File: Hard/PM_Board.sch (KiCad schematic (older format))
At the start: 63 parts, among them J1 Micro_SD_Card_Det_Hirose_DM3AT, J101 LiPo_V+, J102 LiPo_V-, J2 KRC_Conn_SWD, J3 USB_B_Micro, J4 KRC_Conn_CAN, J5 KRC_Conn_CAN, J6 KRC_Conn_CAN, Q1 SSM6J501NU, Q2 2n7002, U1 CY8C58xxLTI-LPxxx, U2 INA226, U3 NCV7342, Y1 24MHz

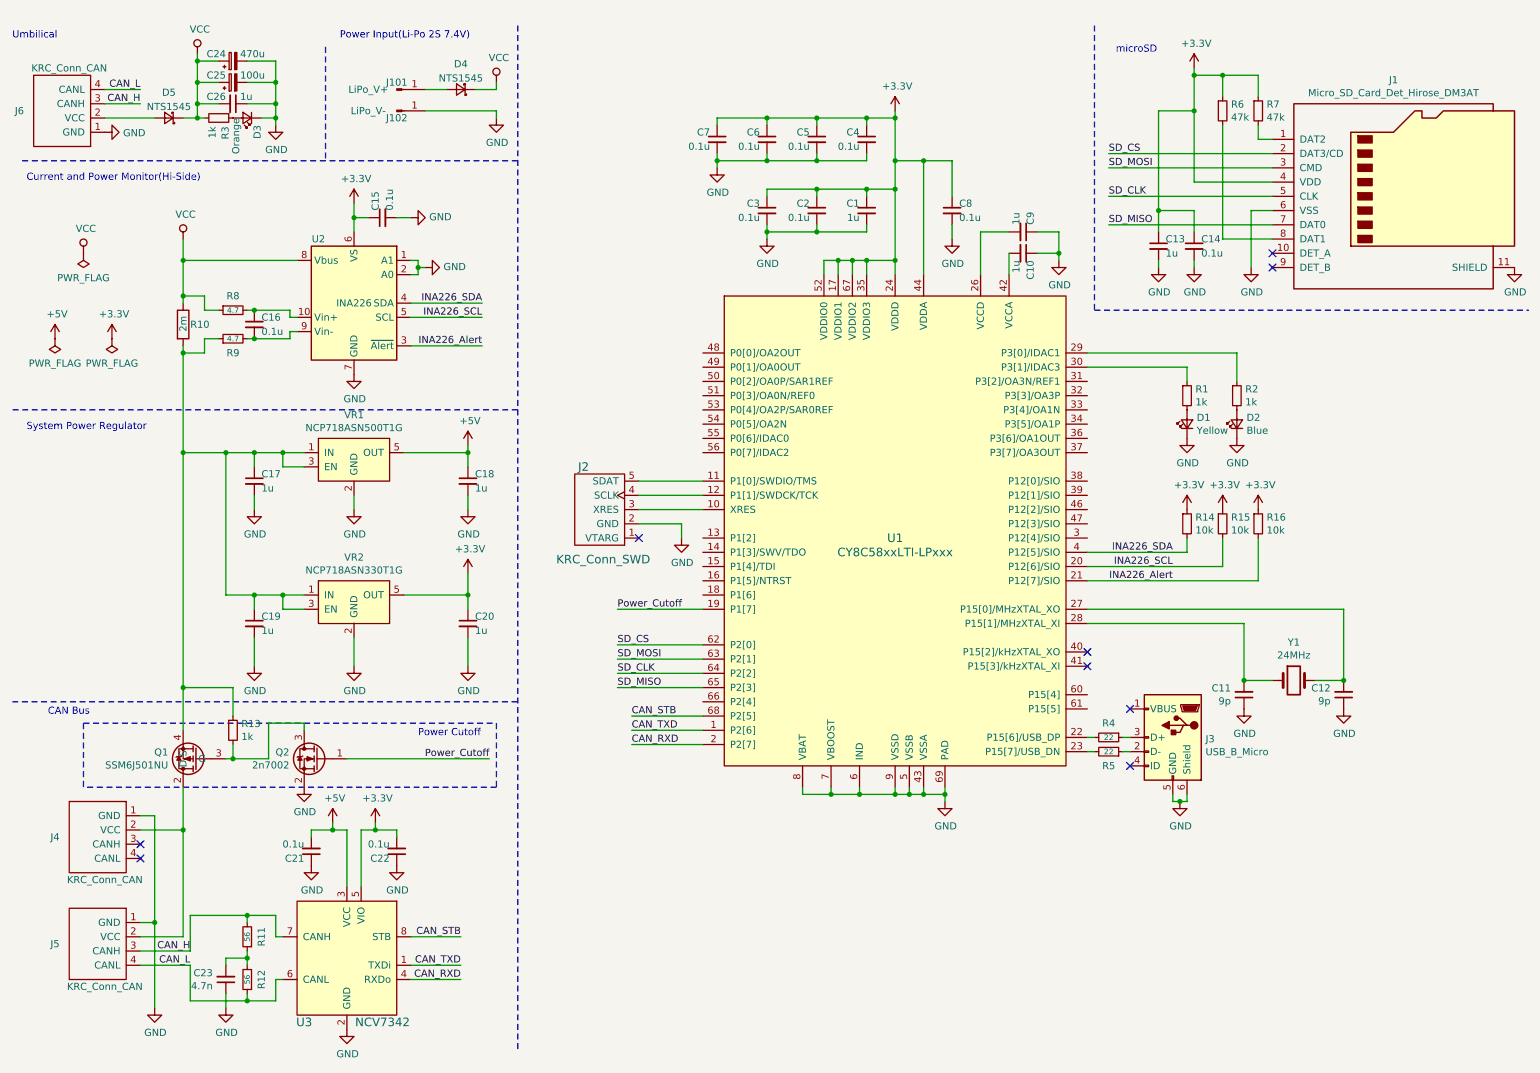
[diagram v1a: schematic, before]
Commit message: [add] 配線中だよ
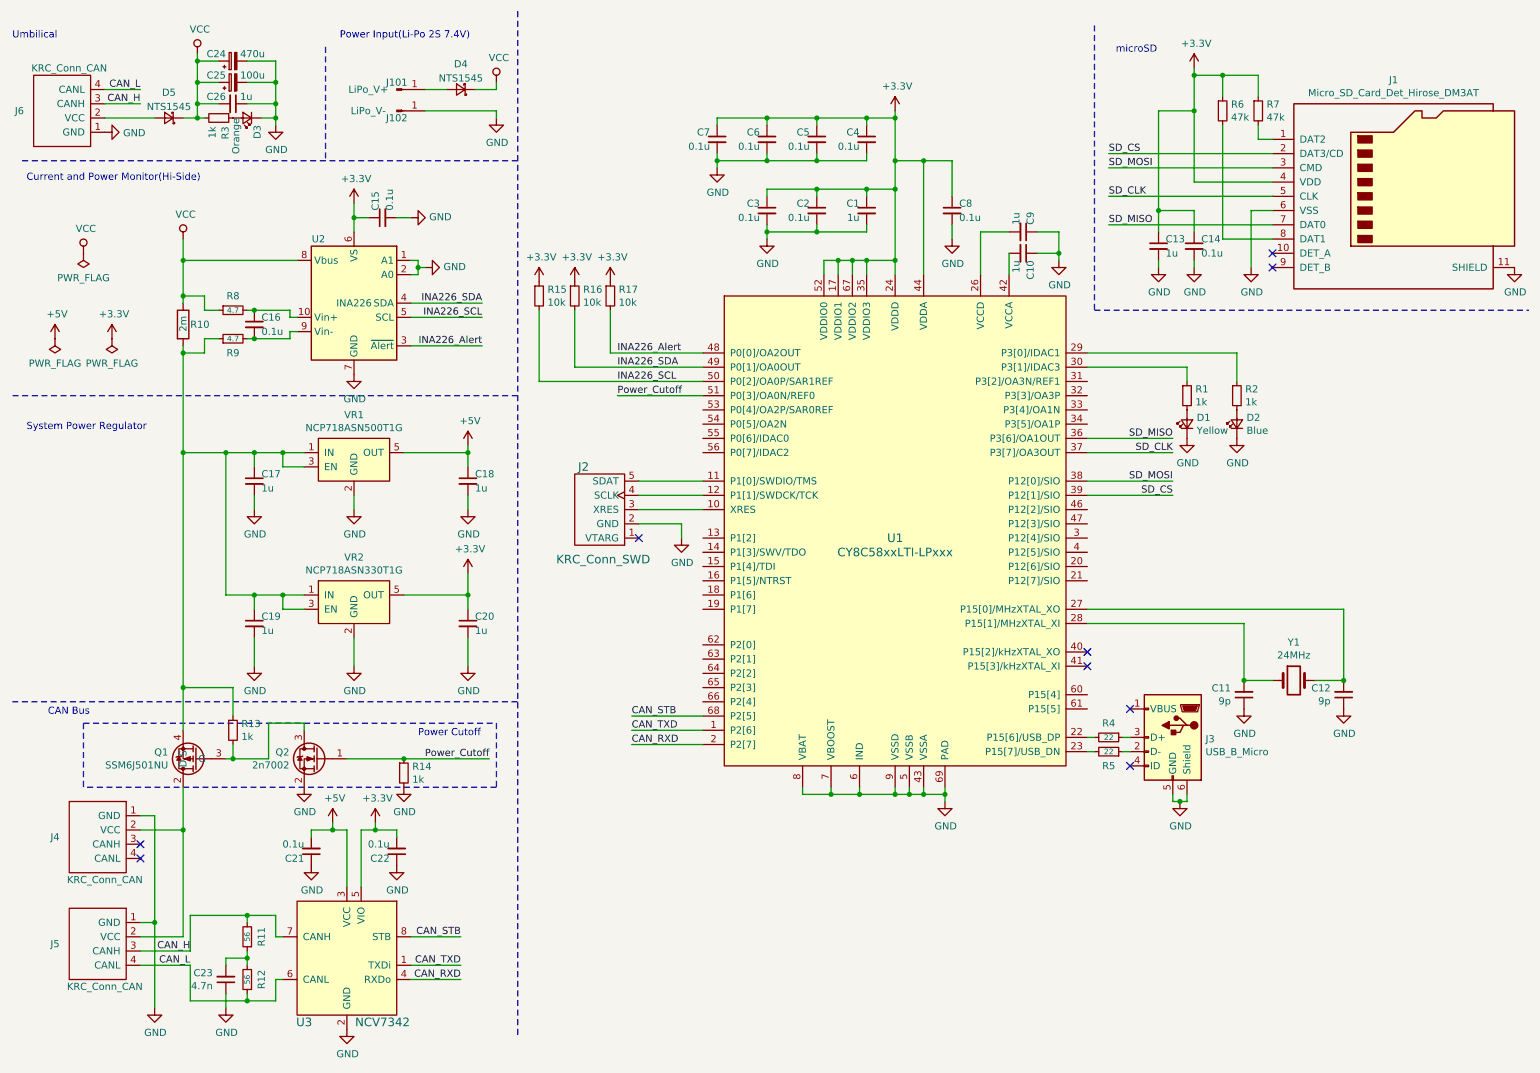
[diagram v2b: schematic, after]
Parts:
- added R14: 1k, Resistor_SMD:R_0402_1005Metric, symbol Device:R_Small
- renumbered R14 to R15, R15 to R16, R16 to R17
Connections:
- net GND: now also R14.2
- net INA226_Alert: now also U1.48 (P0[0]/OA2OUT); no longer U1.21 (P12[7]/SIO)
- net INA226_SCL: now also R15.2, U1.50 (P0[2]/OA0P/SAR1REF); no longer R16.2, U1.20 (P12[6]/SIO)
- net INA226_SDA: now also R16.2, U1.49 (P0[1]/OA0OUT); no longer R15.2, U1.4 (P12[5]/SIO)
- net Power_Cutoff: now also U1.51 (P0[3]/OA0N/REF0), R14.1; no longer U1.19 (P1[7])
- net SD_CLK: now also U1.37 (P3[7]/OA3OUT); no longer U1.64 (P2[2])
- net SD_CS: now also U1.39 (P12[1]/SIO); no longer U1.62 (P2[0])
- net SD_MISO: now also U1.36 (P3[6]/OA1OUT); no longer U1.65 (P2[3])
- net SD_MOSI: now also U1.38 (P12[0]/SIO); no longer U1.63 (P2[1])
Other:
- moved on the sheet: R15, R16, R17
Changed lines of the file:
@@
 	1500 6050 1500 6800
 Wire Notes Line
-	4050 500  4050 7700
+	4050 400  4050 7600
 Wire Notes Line
 	4050 1450 550  1450
@@
 Connection ~ 3700 3500
 Wire Notes Line
-	4050 3200 500  3200
+	4050 3100 500  3100
 Wire Notes Line
 	500  5250 4050 5250
@@
 Wire Wire Line
 	4850 5550 5350 5550
-Text Label 4750 5150 0    50   ~ 0
+Text Label 8650 3400 2    50   ~ 0
 SD_MISO
-Text Label 4750 5050 0    50   ~ 0
+Text Label 8650 3500 2    50   ~ 0
 SD_CLK
-Text Label 4750 4950 0    50   ~ 0
+Text Label 8650 3700 2    50   ~ 0
 SD_MOSI
-Text Label 4750 4850 0    50   ~ 0
+Text Label 8650 3800 2    50   ~ 0
 SD_CS
 Wire Wire Line
-	4750 4850 5350 4850
-Wire Wire Line
-	4750 4950 5350 4950
-Wire Wire Line
-	4750 5050 5350 5050
-Wire Wire Line
-	4750 5150 5350 5150
+	8650 3800 8050 3800
+Wire Wire Line
+	8650 3700 8050 3700
+Wire Wire Line
+	8650 3500 8050 3500
+Wire Wire Line
+	8650 3400 8050 3400
 Text Label 3800 2450 2    50   ~ 0
 INA226_SDA
@@
 Wire Wire Line
 	3300 2550 3800 2550
-Text Label 8650 4200 2    50   ~ 0
+Text Label 4750 2900 0    50   ~ 0
 INA226_SDA
-Text Label 8650 4300 2    50   ~ 0
+Text Label 4750 3000 0    50   ~ 0
 INA226_SCL
-Text Label 8650 4400 2    50   ~ 0
+Text Label 4750 2800 0    50   ~ 0
 INA226_Alert
 Wire Wire Line
-	8050 4200 8750 4200
-Wire Wire Line
-	9000 4300 9000 4100
-Wire Wire Line
-	8050 4300 9000 4300
-Wire Wire Line
-	8750 4100 8750 4200
-Wire Wire Line
-	9250 4400 9250 4100
-Wire Wire Line
-	8050 4400 9250 4400
+	4700 2800 4700 2500
 $Comp
 L power:+3.3V #PWR0137
 U 1 1 5D91E91D
-P 8750 3900
-F 0 "#PWR0137" H 8750 3750 50  0001 C CNN
-F 1 "+3.3V" H 8765 4073 50  0000 C CNN
-F 2 "" H 8750 3900 50  0001 C CNN
-F 3 "" H 8750 3900 50  0001 C CNN
-	1    8750 3900
+P 4200 2300
+F 0 "#PWR0137" H 4200 2150 50  0001 C CNN
+F 1 "+3.3V" H 4215 2473 50  0000 C CNN
+F 2 "" H 4200 2300 50  0001 C CNN
+F 3 "" H 4200 2300 50  0001 C CNN
+	1    4200 2300
 	1    0    0    -1
 $EndComp
@@
 L power:+3.3V #PWR0138
 U 1 1 5D91E993
-P 9000 3900
-F 0 "#PWR0138" H 9000 3750 50  0001 C CNN
-F 1 "+3.3V" H 9015 4073 50  0000 C CNN
-F 2 "" H 9000 3900 50  0001 C CNN
-F 3 "" H 9000 3900 50  0001 C CNN
-	1    9000 3900
+P 4450 2300
+F 0 "#PWR0138" H 4450 2150 50  0001 C CNN
+F 1 "+3.3V" H 4465 2473 50  0000 C CNN
+F 2 "" H 4450 2300 50  0001 C CNN
+F 3 "" H 4450 2300 50  0001 C CNN
+	1    4450 2300
 	1    0    0    -1
 $EndComp
@@
 L power:+3.3V #PWR0139
 U 1 1 5D91EA02
-P 9250 3900
-F 0 "#PWR0139" H 9250 3750 50  0001 C CNN
-F 1 "+3.3V" H 9265 4073 50  0000 C CNN
-F 2 "" H 9250 3900 50  0001 C CNN
-F 3 "" H 9250 3900 50  0001 C CNN
-	1    9250 3900
+P 4700 2300
+F 0 "#PWR0139" H 4700 2150 50  0001 C CNN
+F 1 "+3.3V" H 4715 2473 50  0000 C CNN
+F 2 "" H 4700 2300 50  0001 C CNN
+F 3 "" H 4700 2300 50  0001 C CNN
+	1    4700 2300
 	1    0    0    -1
 $EndComp
@@
 Wire Wire Line
 	6900 1450 7100 1450
-Text Label 4750 4600 0    50   ~ 0
+Text Label 4750 3100 0    50   ~ 0
 Power_Cutoff
 Wire Wire Line
-	4750 4600 5350 4600
+	4750 3100 5350 3100
 $Comp
 L Device:R R10
@@
 	3900 1100 3400 1100
 $Comp
-L Device:R_Small R14
+L Device:R_Small R15
 U 1 1 5DECB132
-P 8750 4000
-F 0 "R14" H 8809 4046 50  0000 L CNN
-F 1 "10k" H 8809 3955 50  0000 L CNN
-F 2 "Resistor_SMD:R_0402_1005Metric" H 8750 4000 50  0001 C CNN
-F 3 "https://b2b-api.panasonic.eu/file_stream/pids/fileversion/1242" H 8750 4000 50  0001 C CNN
-F 4 "Digikey" H 8750 4000 50  0001 C CNN "Agency"
-F 5 "ERJ-2GEJ103X" H 8750 4000 50  0001 C CNN "MPN"
-F 6 "https://www.digikey.jp/product-detail/ja/panasonic-electronic-components/ERJ-2GEJ103X/P10KJCT-ND/146734" H 8750 4000 50  0001 C CNN "Link"
-F 7 "10kΩ" H 8750 4000 50  0001 C CNN "Value"
-	1    8750 4000
+P 4200 2400
+F 0 "R15" H 4259 2446 50  0000 L CNN
+F 1 "10k" H 4259 2355 50  0000 L CNN
+F 2 "Resistor_SMD:R_0402_1005Metric" H 4200 2400 50  0001 C CNN
+F 3 "https://b2b-api.panasonic.eu/file_stream/pids/fileversion/1242" H 4200 2400 50  0001 C CNN
+F 4 "Digikey" H 4200 2400 50  0001 C CNN "Agency"
+F 5 "ERJ-2GEJ103X" H 4200 2400 50  0001 C CNN "MPN"
+F 6 "https://www.digikey.jp/product-detail/ja/panasonic-electronic-components/ERJ-2GEJ103X/P10KJCT-ND/146734" H 4200 2400 50  0001 C CNN "Link"
+F 7 "10kΩ" H 4200 2400 50  0001 C CNN "Value"
+	1    4200 2400
 	1    0    0    -1
 $EndComp
@@
 $EndComp
 $Comp
-L Device:R_Small R15
+L Device:R_Small R16
 U 1 1 5DEF321A
-P 9000 4000
-F 0 "R15" H 9059 4046 50  0000 L CNN
-F 1 "10k" H 9059 3955 50  0000 L CNN
-F 2 "Resistor_SMD:R_0402_1005Metric" H 9000 4000 50  0001 C CNN
-F 3 "https://b2b-api.panasonic.eu/file_stream/pids/fileversion/1242" H 9000 4000 50  0001 C CNN
-F 4 "Digikey" H 9000 4000 50  0001 C CNN "Agency"
-F 5 "ERJ-2GEJ103X" H 9000 4000 50  0001 C CNN "MPN"
-F 6 "https://www.digikey.jp/product-detail/ja/panasonic-electronic-components/ERJ-2GEJ103X/P10KJCT-ND/146734" H 9000 4000 50  0001 C CNN "Link"
-F 7 "10kΩ" H 9000 4000 50  0001 C CNN "Value"
-	1    9000 4000
-	1    0    0    -1
-$EndComp
-$Comp
-L Device:R_Small R16
+P 4450 2400
+F 0 "R16" H 4509 2446 50  0000 L CNN
+F 1 "10k" H 4509 2355 50  0000 L CNN
+F 2 "Resistor_SMD:R_0402_1005Metric" H 4450 2400 50  0001 C CNN
+F 3 "https://b2b-api.panasonic.eu/file_stream/pids/fileversion/1242" H 4450 2400 50  0001 C CNN
+F 4 "Digikey" H 4450 2400 50  0001 C CNN "Agency"
+F 5 "ERJ-2GEJ103X" H 4450 2400 50  0001 C CNN "MPN"
+F 6 "https://www.digikey.jp/product-detail/ja/panasonic-electronic-components/ERJ-2GEJ103X/P10KJCT-ND/146734" H 4450 2400 50  0001 C CNN "Link"
+F 7 "10kΩ" H 4450 2400 50  0001 C CNN "Value"
+	1    4450 2400
+	1    0    0    -1
+$EndComp
+$Comp
+L Device:R_Small R17
 U 1 1 5DEF32AE
-P 9250 4000
-F 0 "R16" H 9309 4046 50  0000 L CNN
-F 1 "10k" H 9309 3955 50  0000 L CNN
-F 2 "Resistor_SMD:R_0402_1005Metric" H 9250 4000 50  0001 C CNN
-F 3 "https://b2b-api.panasonic.eu/file_stream/pids/fileversion/1242" H 9250 4000 50  0001 C CNN
-F 4 "Digikey" H 9250 4000 50  0001 C CNN "Agency"
-F 5 "ERJ-2GEJ103X" H 9250 4000 50  0001 C CNN "MPN"
-F 6 "https://www.digikey.jp/product-detail/ja/panasonic-electronic-components/ERJ-2GEJ103X/P10KJCT-ND/146734" H 9250 4000 50  0001 C CNN "Link"
-F 7 "10kΩ" H 9250 4000 50  0001 C CNN "Value"
-	1    9250 4000
+P 4700 2400
+F 0 "R17" H 4759 2446 50  0000 L CNN
+F 1 "10k" H 4759 2355 50  0000 L CNN
+F 2 "Resistor_SMD:R_0402_1005Metric" H 4700 2400 50  0001 C CNN
+F 3 "https://b2b-api.panasonic.eu/file_stream/pids/fileversion/1242" H 4700 2400 50  0001 C CNN
+F 4 "Digikey" H 4700 2400 50  0001 C CNN "Agency"
+F 5 "ERJ-2GEJ103X" H 4700 2400 50  0001 C CNN "MPN"
+F 6 "https://www.digikey.jp/product-detail/ja/panasonic-electronic-components/ERJ-2GEJ103X/P10KJCT-ND/146734" H 4700 2400 50  0001 C CNN "Link"
+F 7 "10kΩ" H 4700 2400 50  0001 C CNN "Value"
+	1    4700 2400
 	1    0    0    -1
 $EndComp
@@
 $EndComp
 Wire Wire Line
-	2850 5650 3850 5650
+	2850 5650 3250 5650
 Wire Wire Line
 	1700 3500 1700 5150
@@
 Wire Wire Line
 	1700 5150 1700 5450
+$Comp
+L Device:R_Small R14
+U 1 1 5DD77184
+P 3250 5750
+F 0 "R14" H 3309 5796 50  0000 L CNN
+F 1 "1k" H 3309 5705 50  0000 L CNN
+F 2 "Resistor_SMD:R_0402_1005Metric" H 3250 5750 50  0001 C CNN
+F 3 "https://b2b-api.panasonic.eu/file_stream/pids/fileversion/1242" H 3250 5750 50  0001 C CNN
+F 4 "Digikey" H 3250 5750 50  0001 C CNN "Agency"
+F 5 "ERJ-2GEJ102X" H 3250 5750 50  0001 C CNN "MPN"
+F 6 "https://www.digikey.jp/product-detail/ja/panasonic-electronic-components/ERJ-2GEJ102X/P1.0KJCT-ND/146897" H 3250 5750 50  0001 C CNN "Link"
+F 7 "1kΩ" H 3250 5750 50  0001 C CNN "Value"
+	1    3250 5750
+	1    0    0    -1
+$EndComp
+Connection ~ 3250 5650
+Wire Wire Line
+	3250 5650 3850 5650
+$Comp
+L power:GND #PWR0148
+U 1 1 5DD77234
+P 3250 5850
+F 0 "#PWR0148" H 3250 5600 50  0001 C CNN
+F 1 "GND" H 3255 5677 50  0000 C CNN
+F 2 "" H 3250 5850 50  0001 C CNN
+F 3 "" H 3250 5850 50  0001 C CNN
+	1    3250 5850
+	1    0    0    -1
+$EndComp
+Wire Wire Line
+	4450 2500 4450 2900
+Wire Wire Line
+	4450 2900 5350 2900
+Wire Wire Line
+	4200 2500 4200 3000
+Wire Wire Line
+	4200 3000 5350 3000
+Wire Wire Line
+	4700 2800 5350 2800
 $EndSCHEMATC
